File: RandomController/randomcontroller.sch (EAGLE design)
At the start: 103 parts, among them IC1 TPS2054B, IC2 TPS2054B, IC3 TPS2054B, IC4 TPS2054B, IC6 PIC16F1939PT, Q1 NX-3215, U1 MCP1700_SOT23

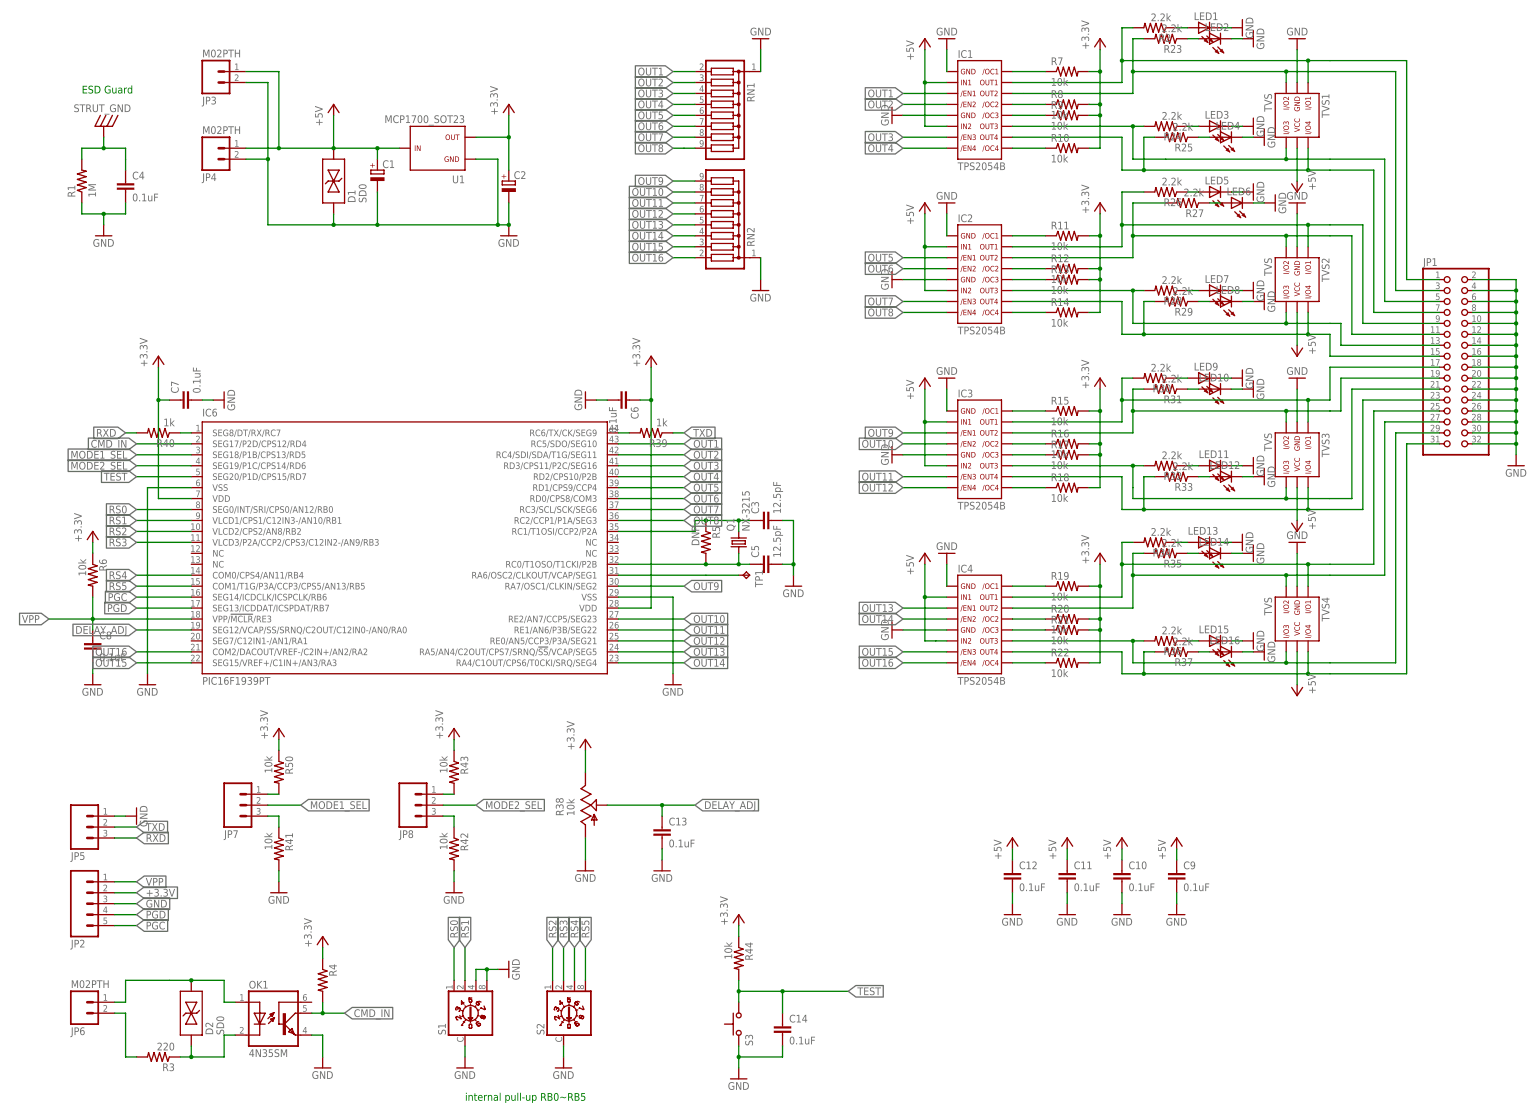
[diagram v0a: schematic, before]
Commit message: random controller first version
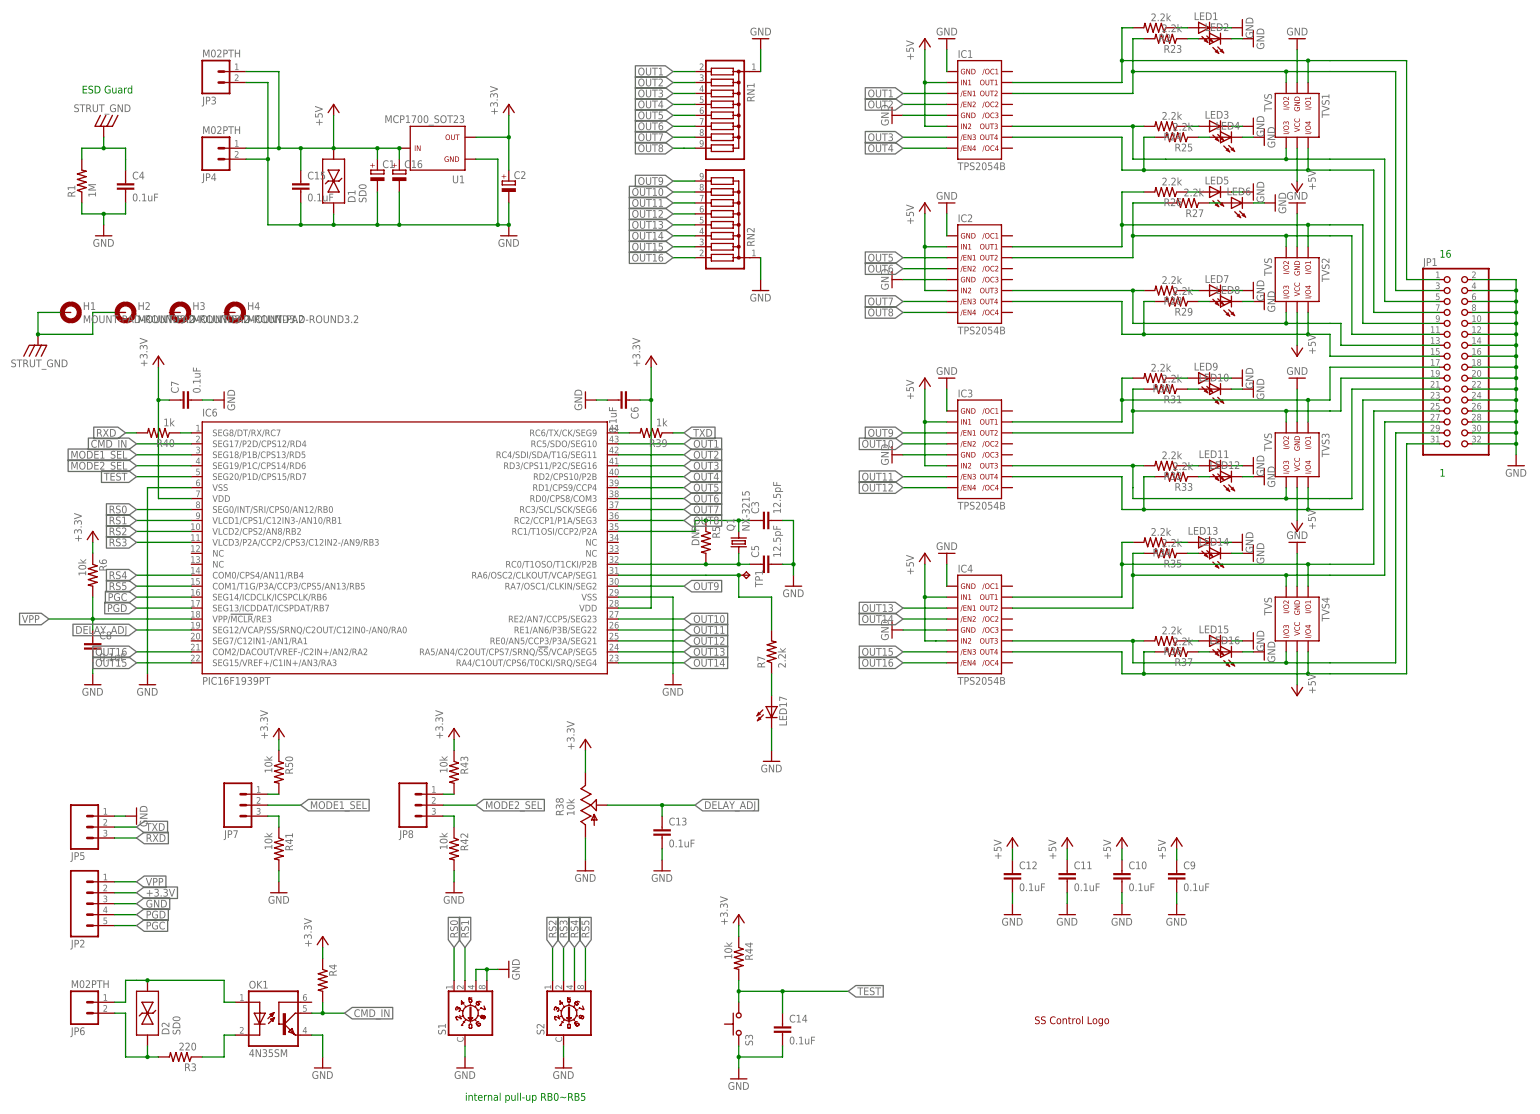
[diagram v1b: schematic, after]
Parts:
- removed R10, R11, R12, R13, R14, R15, R16, R17, R18, R19, R20, R21, R22, R8, R9: 10k, WaterDrop:R0805(2012)
- added C15: 0.1uF, WaterDrop:C0805(2012)
- added C16: (no value), yBrainDigital:C-TANTAL-A
- added H1, H2, H3, H4: MOUNT-PAD-ROUND3.2, holes:MOUNT-PAD-ROUND3.2
- added LED17: (no value), adafruit:LEDCHIPLED_0805
- added U$1: LOGO, WaterDrop:LOGO
- R7: value 10k -> 2.2k
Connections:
- removed net N$33: IC1.P$13, R8.1
- removed net N$34: IC1.P$12, R9.1
- removed net N$35: IC1.P$9, R10.1
- removed net N$36: IC2.P$16, R11.1
- removed net N$37: IC2.P$13, R12.1
- removed net N$38: IC2.P$12, R13.1
- removed net N$39: IC2.P$9, R14.1
- removed net N$40: IC3.P$16, R15.1
- removed net N$41: IC3.P$13, R16.1
- removed net N$42: IC3.P$12, R17.1
- removed net N$43: IC3.P$9, R18.1
- removed net N$44: IC4.P$16, R19.1
- removed net N$45: IC4.P$13, R20.1
- removed net N$46: IC4.P$12, R21.1
- removed net N$47: IC4.P$9, R22.1
- net +3.3V: no longer R10.2, R11.2, R12.2, R13.2, R14.2, R15.2, R16.2, R17.2, R18.2, R19.2, R20.2, R21.2, R22.2, R7.2, R8.2, R9.2
- net +5V: now also C15.1, C16.+
- net CLKOUT: now also R7.2
- net GND: now also C15.2, C16.-, LED17.C
- net N$3: no longer D2.P$1
- net N$32: now also LED17.A; no longer IC1.P$16
- net N$4: now also D2.P$1
- net STRUT_GND: now also H1.MOUNT, H2.MOUNT
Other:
- note added: "1"
- note added: "16"
- moved on the sheet: D2, R3, R7
